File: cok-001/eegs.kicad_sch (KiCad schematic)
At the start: 40 parts

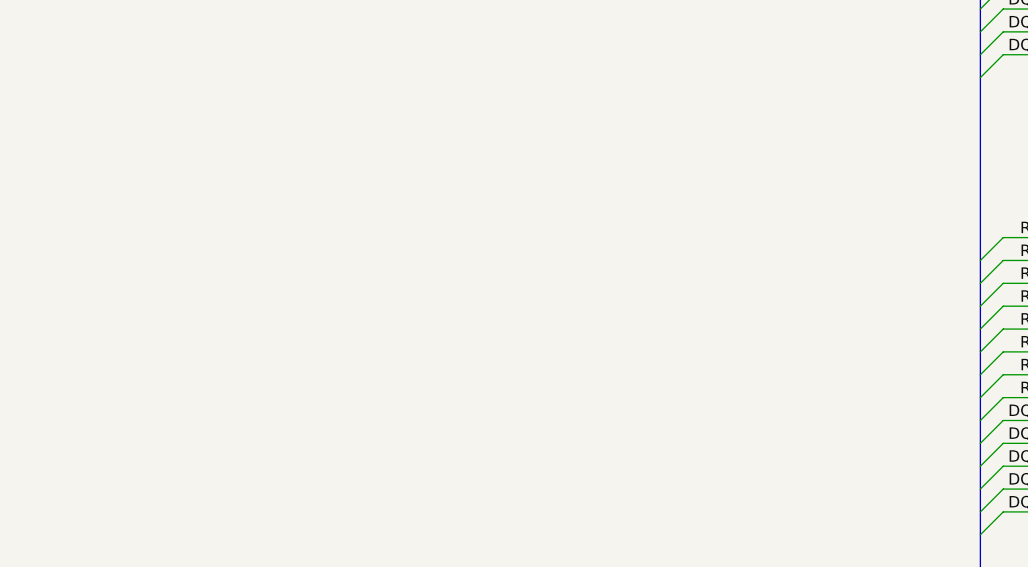
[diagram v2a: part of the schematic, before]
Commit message: footprints
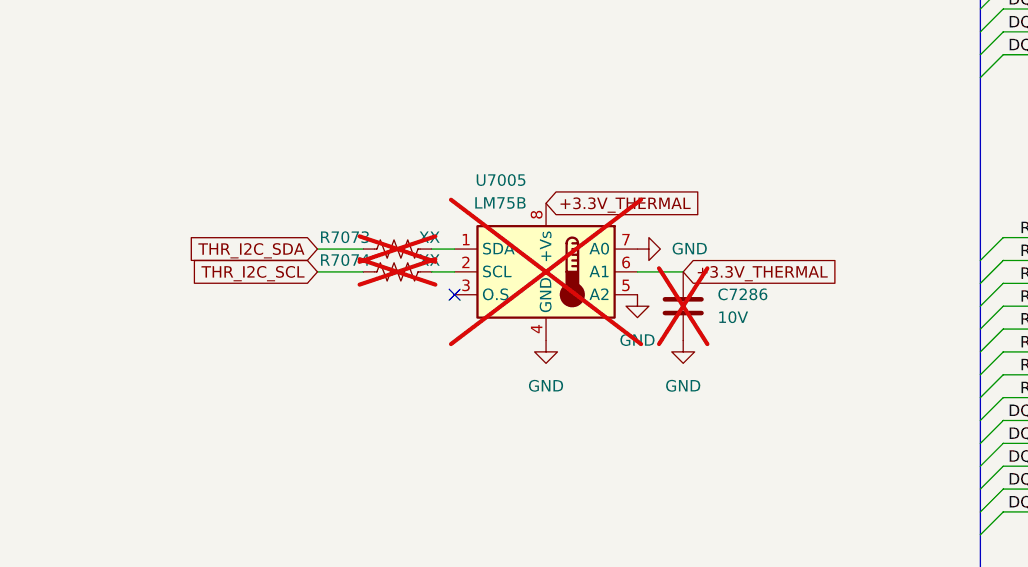
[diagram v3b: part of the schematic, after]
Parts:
- added C7286: 10V, Capacitor_SMD:C_0402_1005Metric, symbol Device:C
- added R7073, R7074: XX, Resistor_SMD:R_0402_1005Metric, symbol Device:R_US
- added U7005: LM75B, Package_SO:VSSOP-8_3x3mm_P0.65mm, symbol Sensor_Temperature:LM75B
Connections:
- net GND: now also C7286.2, U7005.4 (GND), U7005.5 (A2), U7005.7 (A0)
- new net: R7073.2, U7005.1 (SDA)
- new net: R7074.2, U7005.2 (SCL)
- new net +3.3V_THERMAL: C7286.1, U7005.6 (A1), U7005.8 (+Vs)
- new net THR_I2C_SCL: R7074.1
- new net THR_I2C_SDA: R7073.1
- no-connect marks 74 -> 75

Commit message: ps2
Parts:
- added R7033: 0, Resistor_SMD:R_0603_1608Metric, symbol Device:R_US
- added R7034: 47, Resistor_SMD:R_0402_1005Metric, symbol Device:R_US
- added R7044, R7045: 1k, Resistor_SMD:R_0603_1608Metric, symbol Device:R_US
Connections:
- net GND: now also U7004.T29 (DQBA8), R7033.1
- net at U7004.A5 (~{INTIN1}): now also R7034.2
- net at U7004.AA1 (CLKGCCG): now also R7033.2
- net CFMN_B: now reaches U7004.AA30 (CFMNB)
- net CFMN_B: now also U7003.D7 (CFMN)
- net CFM_B: now reaches U7004.AA32 (CFMB)
- net CFM_B: now also U7003.C7 (CFM)
- net CTM_B: now reaches U7004.AB30 (CTMB)
- net CTM_B: now also U7003.E1 (CTM)
- net CTMN_B: now reaches U7004.AB32 (CTMNB)
- net CTMN_B: now also U7003.D1 (CTMN)
- net at U7004.AL11 (~{INT}): now also R7034.1
- net at U7004.B4 (~{ERESET}): now also R7044.1
- net CFM_A: now reaches U7004.G30 (CFMA)
- net CFM_A: now also U7002.C7 (CFM)
- net CFMN_A: now reaches U7004.G32 (CFMNA)
- net CFMN_A: now also U7002.D7 (CFMN)
- net CTMN_A: now reaches U7004.H30 (CTMNA)
- net CTMN_A: now also U7002.E1 (CTM)
- net CTM_A: now reaches U7004.H32 (CTMA)
- net CTM_A: now also U7002.D1 (CTMN)
- net at U7004.Y1 (PwrUp): now also R7045.1
- new net PWRUP_EE: R7045.2
- new net ~{EGRST}: R7044.2
- no-connect marks 75 -> 76
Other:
- moved on the sheet: C7286, R7073, R7074, U7002, U7005

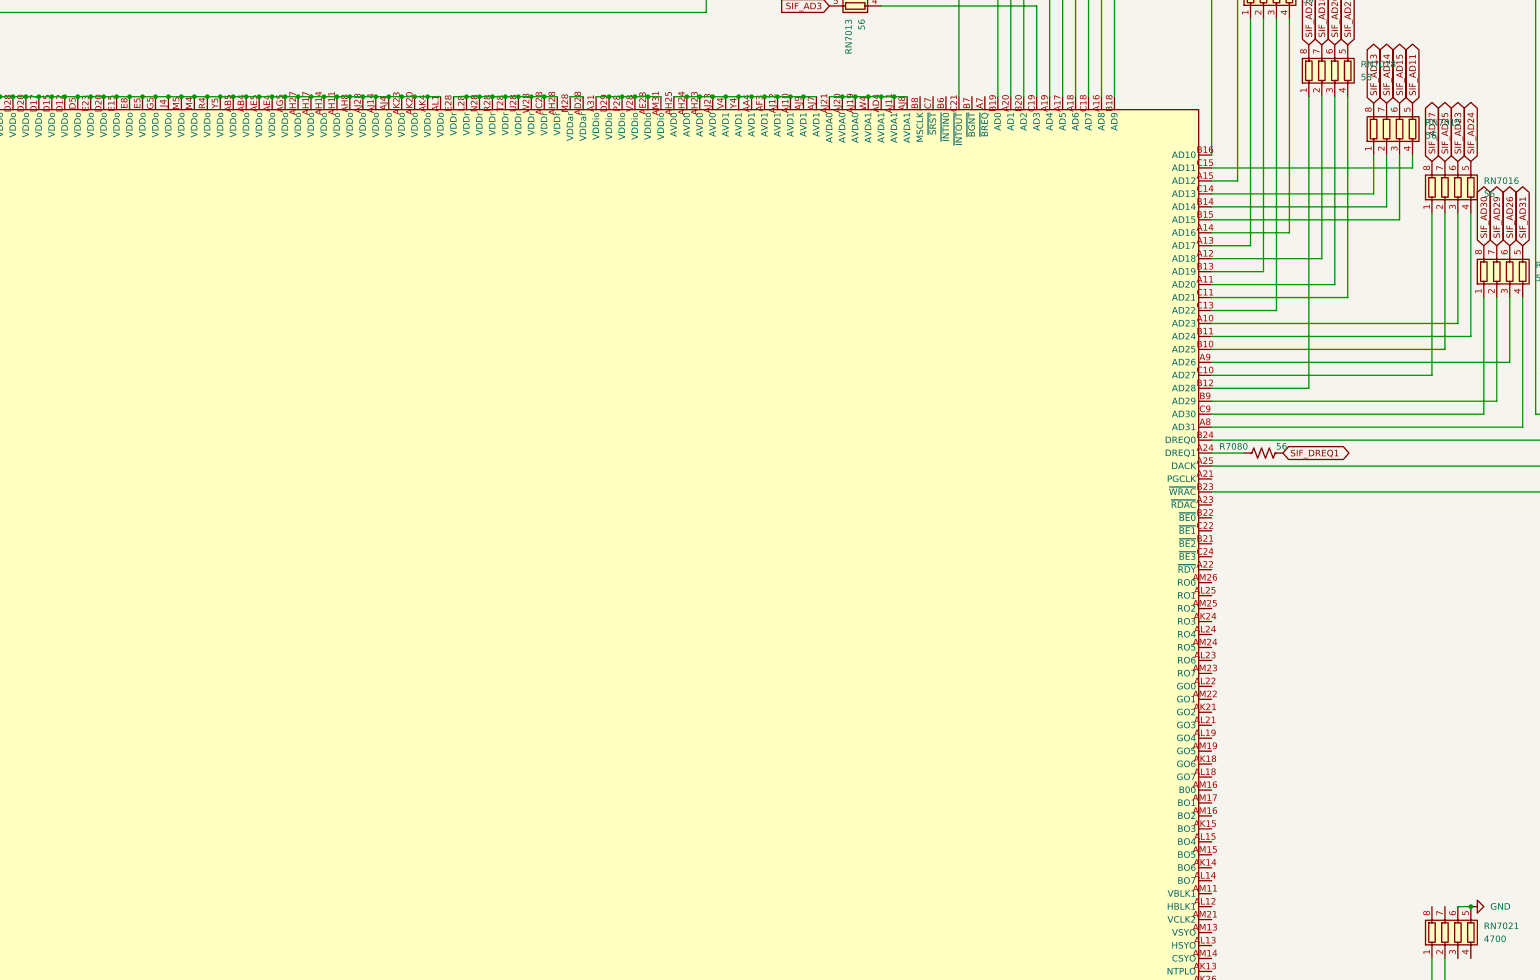
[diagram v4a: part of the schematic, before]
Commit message: PCIe
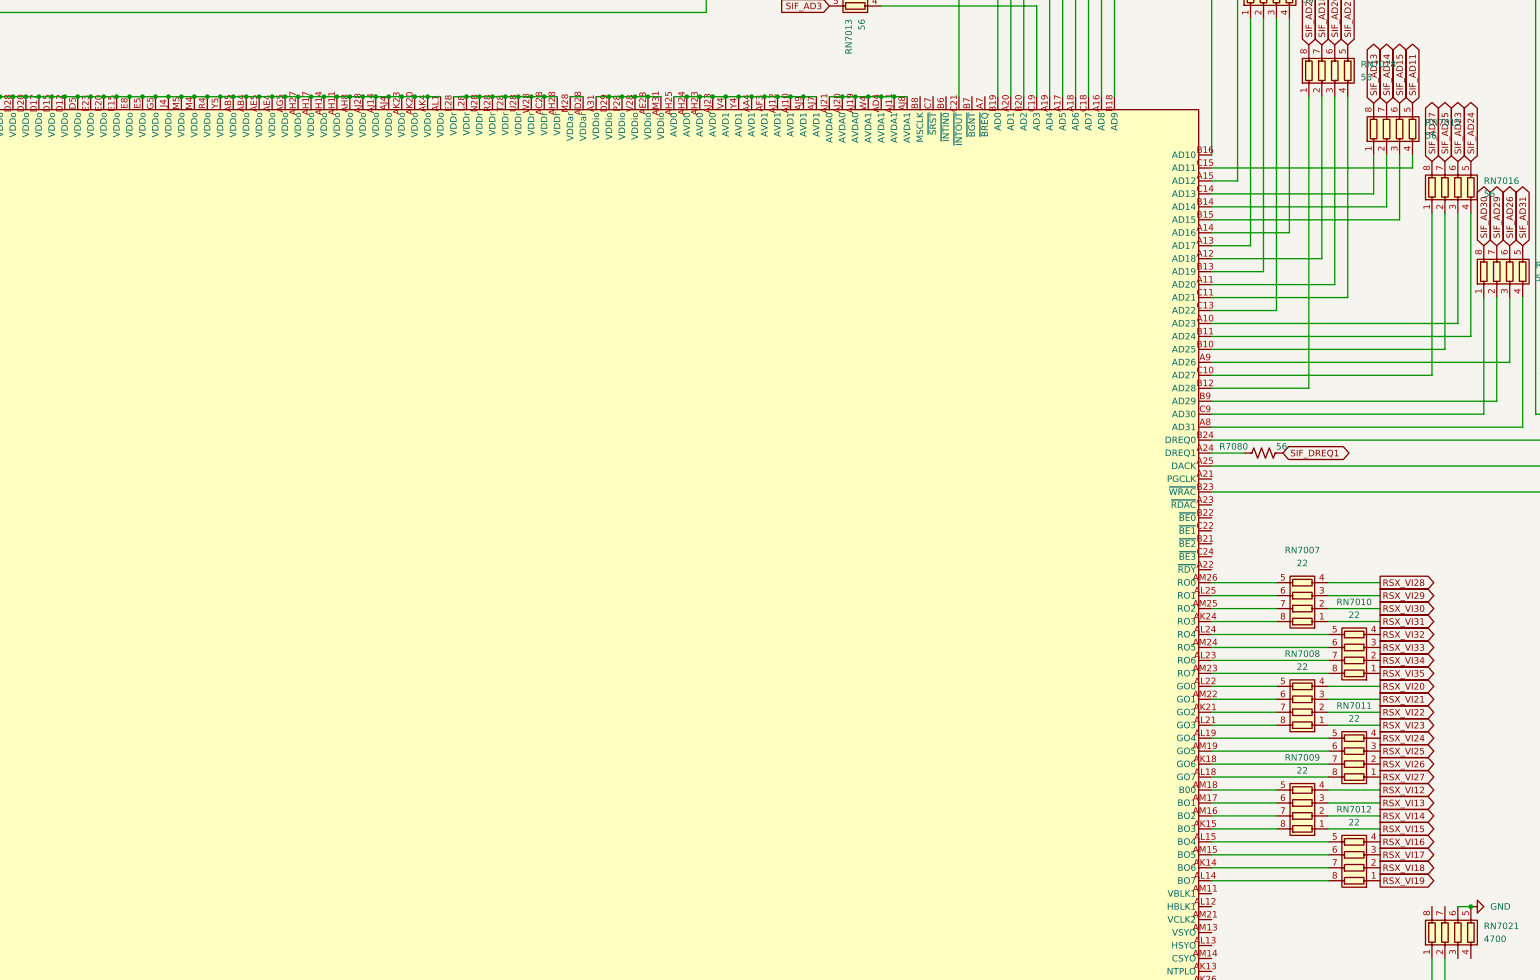
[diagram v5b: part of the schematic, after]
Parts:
- added RN7007, RN7008, RN7009, RN7010, RN7011, RN7012: 22, Resistor_SMD:R_Array_Convex_4x0402, symbol Device:R_Pack04
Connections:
- net at U7004.AB4 (VDDo), U7004.AB5 (VDDo), U7004.AE4 (VDDo)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: now also U7004.E20 (VDDo)
- net at U7004.AK14 (BO6): now also RN7012.7 (R2.2)
- net at U7004.AK15 (BO3): now also RN7009.8 (R1.2)
- net at U7004.AK18 (GO6): now also RN7011.7 (R2.2)
- net at U7004.AK21 (GO2): now also RN7008.7 (R2.2)
- net at U7004.AK24 (RO3): now also RN7007.8 (R1.2)
- net at U7004.AL14 (BO7): now also RN7012.8 (R1.2)
- net at U7004.AL15 (BO4): now also RN7012.5 (R4.2)
- net at U7004.AL18 (GO7): now also RN7011.8 (R1.2)
- net at U7004.AL19 (GO4): now also RN7011.5 (R4.2)
- net at U7004.AL21 (GO3): now also RN7008.8 (R1.2)
- net at U7004.AL22 (GO0): now also RN7008.5 (R4.2)
- net at U7004.AL23 (RO6): now also RN7010.7 (R2.2)
- net at U7004.AL24 (RO4): now also RN7010.5 (R4.2)
- net at U7004.AL25 (RO1): now also RN7007.6 (R3.2)
- net at U7004.AM15 (BO5): now also RN7012.6 (R3.2)
- net at U7004.AM16 (BO2): now also RN7009.7 (R2.2)
- net at U7004.AM17 (BO1): now also RN7009.6 (R3.2)
- net at U7004.AM19 (GO5): now also RN7011.6 (R3.2)
- net at U7004.AM22 (GO1): now also RN7008.6 (R3.2)
- net at U7004.AM23 (RO7): now also RN7010.8 (R1.2)
- net at U7004.AM24 (RO5): now also RN7010.6 (R3.2)
- net at U7004.AM25 (RO2): now also RN7007.7 (R2.2)
- net at U7004.AM26 (RO0): now also RN7007.5 (R4.2)
- new net: RN7009.5 (R4.2), U7004.AM18 (B00)
- new net RSX_VI12: RN7009.4 (R4.1)
- new net RSX_VI13: RN7009.3 (R3.1)
- new net RSX_VI14: RN7009.2 (R2.1)
- new net RSX_VI15: RN7009.1 (R1.1)
- new net RSX_VI16: RN7012.4 (R4.1)
- new net RSX_VI17: RN7012.3 (R3.1)
- new net RSX_VI18: RN7012.2 (R2.1)
- new net RSX_VI19: RN7012.1 (R1.1)
- new net RSX_VI20: RN7008.4 (R4.1)
- new net RSX_VI21: RN7008.3 (R3.1)
- new net RSX_VI22: RN7008.2 (R2.1)
- new net RSX_VI23: RN7008.1 (R1.1)
- new net RSX_VI24: RN7011.4 (R4.1)
- new net RSX_VI25: RN7011.3 (R3.1)
- new net RSX_VI26: RN7011.2 (R2.1)
- new net RSX_VI27: RN7011.1 (R1.1)
- new net RSX_VI28: RN7007.4 (R4.1)
- new net RSX_VI29: RN7007.3 (R3.1)
- new net RSX_VI30: RN7007.2 (R2.1)
- new net RSX_VI31: RN7007.1 (R1.1)
- new net RSX_VI32: RN7010.4 (R4.1)
- new net RSX_VI33: RN7010.3 (R3.1)
- new net RSX_VI34: RN7010.2 (R2.1)
- new net RSX_VI35: RN7010.1 (R1.1)
